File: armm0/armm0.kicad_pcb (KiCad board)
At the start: 2 copper layers, 25.4 x 52.1 mm, 20 parts, among them J1 Conn_02x10_Odd_Even, J4 Conn_02x08_Odd_Even, J5 Conn_02x08_Odd_Even, J6 Conn_01x05_Male, J7 Conn_01x05_Male, J8 Conn_01x03_Male, U1 STM32F070F6Px, U2 LD1117S33TR_SOT223

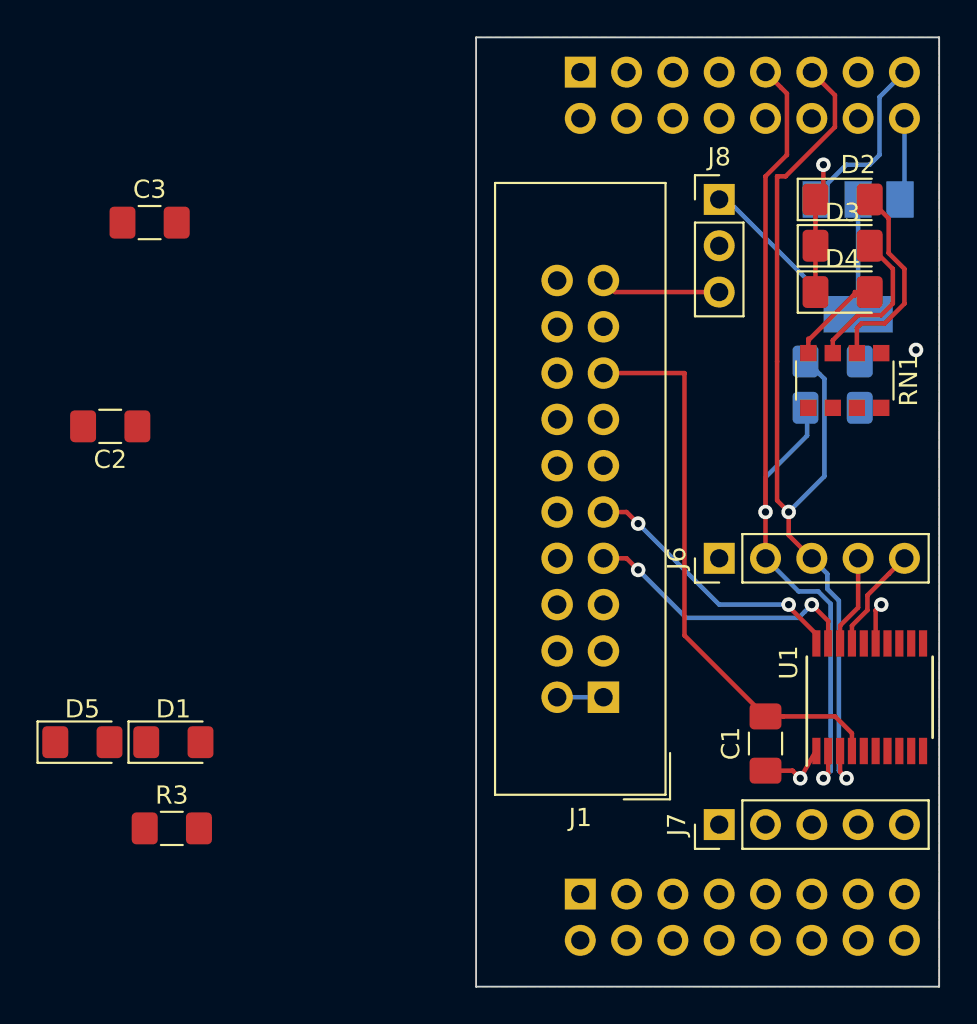
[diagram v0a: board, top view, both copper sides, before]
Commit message: pcb: All connected
Signed-off-by: Ben Lancaster <bdl@live.co.uk>
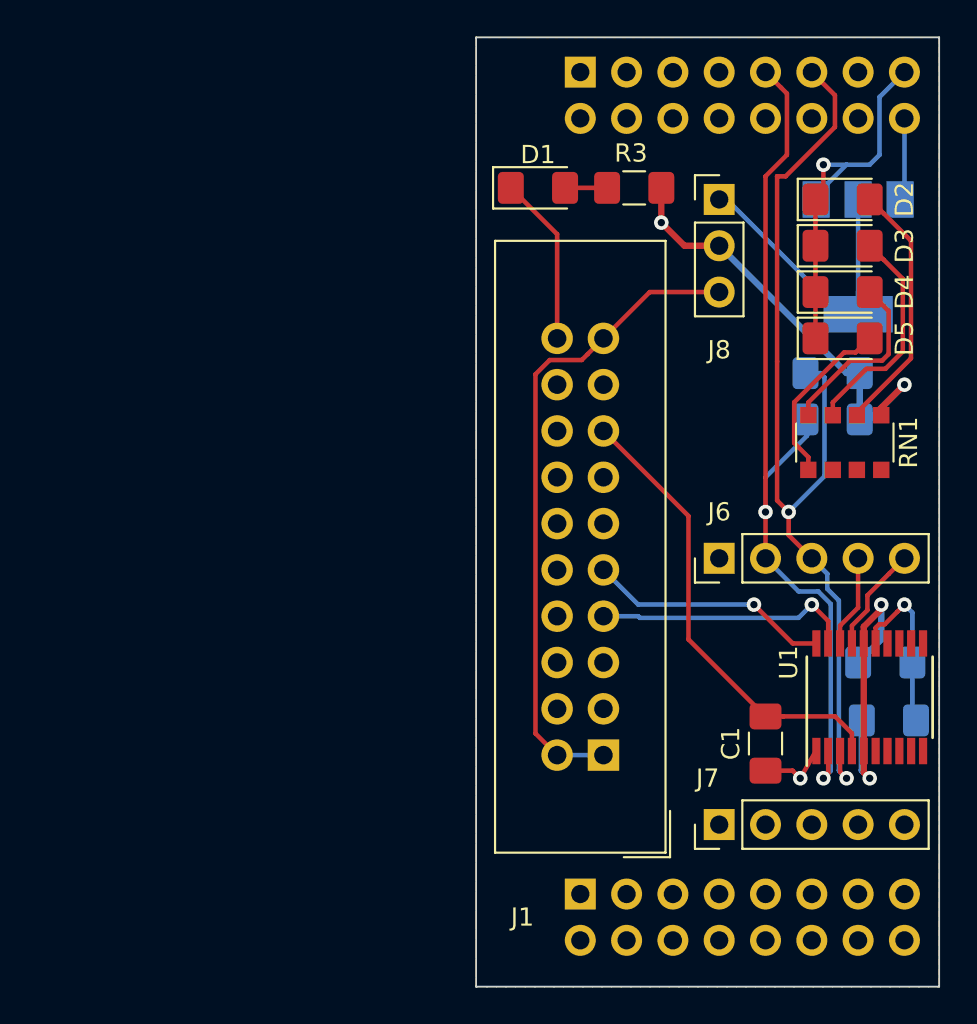
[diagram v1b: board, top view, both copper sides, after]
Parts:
- C2, C3: moved to B.Cu
- moved D5 47.2 mm to (95.0, 47.6)
- moved C3 47.0 mm to (97.4, 65.4)
- moved C2 45.7 mm to (97.6, 68.6), turned to 0 degrees
- moved R3 43.3 mm to (83.6, 39.4), turned to 180 degrees
- moved D1 36.4 mm to (78.3, 39.4)
- moved RN1 3.41 mm to (95.2, 53.3)
- moved J1 3.17 mm to (81.9, 70.5)
- moved R1 0.63 mm to (94.5, 52.1)
- moved R2 0.63 mm to (94.5, 49.5)
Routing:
- net +3V3: track 0.00 -> 41.3 mm, vias 1 -> 4
- net STLINK_3V3: track 9.15 -> 35.9 mm
- net GND: track 23.3 -> 44.1 mm
- net Net-(D5-Pad2): track 0.00 -> 9.62 mm
- net NRST: track 31.2 -> 25.4 mm
- net Net-(D4-Pad2): track 5.36 -> 10.0 mm
- net Net-(D3-Pad2): track 8.53 -> 12.3 mm
- net Net-(D2-Pad2): track 11.0 -> 14.0 mm
- net Net-(D1-Pad2): track 0.00 -> 2.30 mm
- net SWDIO: track 15.6 -> 14.3 mm, vias 2 -> 1
- net SWCLK: track 15.0 -> 13.9 mm, vias 2 -> 1
